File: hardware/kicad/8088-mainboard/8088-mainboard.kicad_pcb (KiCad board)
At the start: 2 copper layers, 149 x 90 mm, 62 parts, among them J1 Exp0, J2 POWER 5v, J3 Exp1, J4 Exp2, SW1 Reset, U1 8088, U10 74LS273, U11 74LS00, U12 74LS138, U13 HM62256BLP, U2 8284, U3 74LS373, U4 74LS373, U5 74LS245, U6 8288, U7 74LS138, U8 28C256, U9 HM62256BLP, Y1 14.31818 MHz

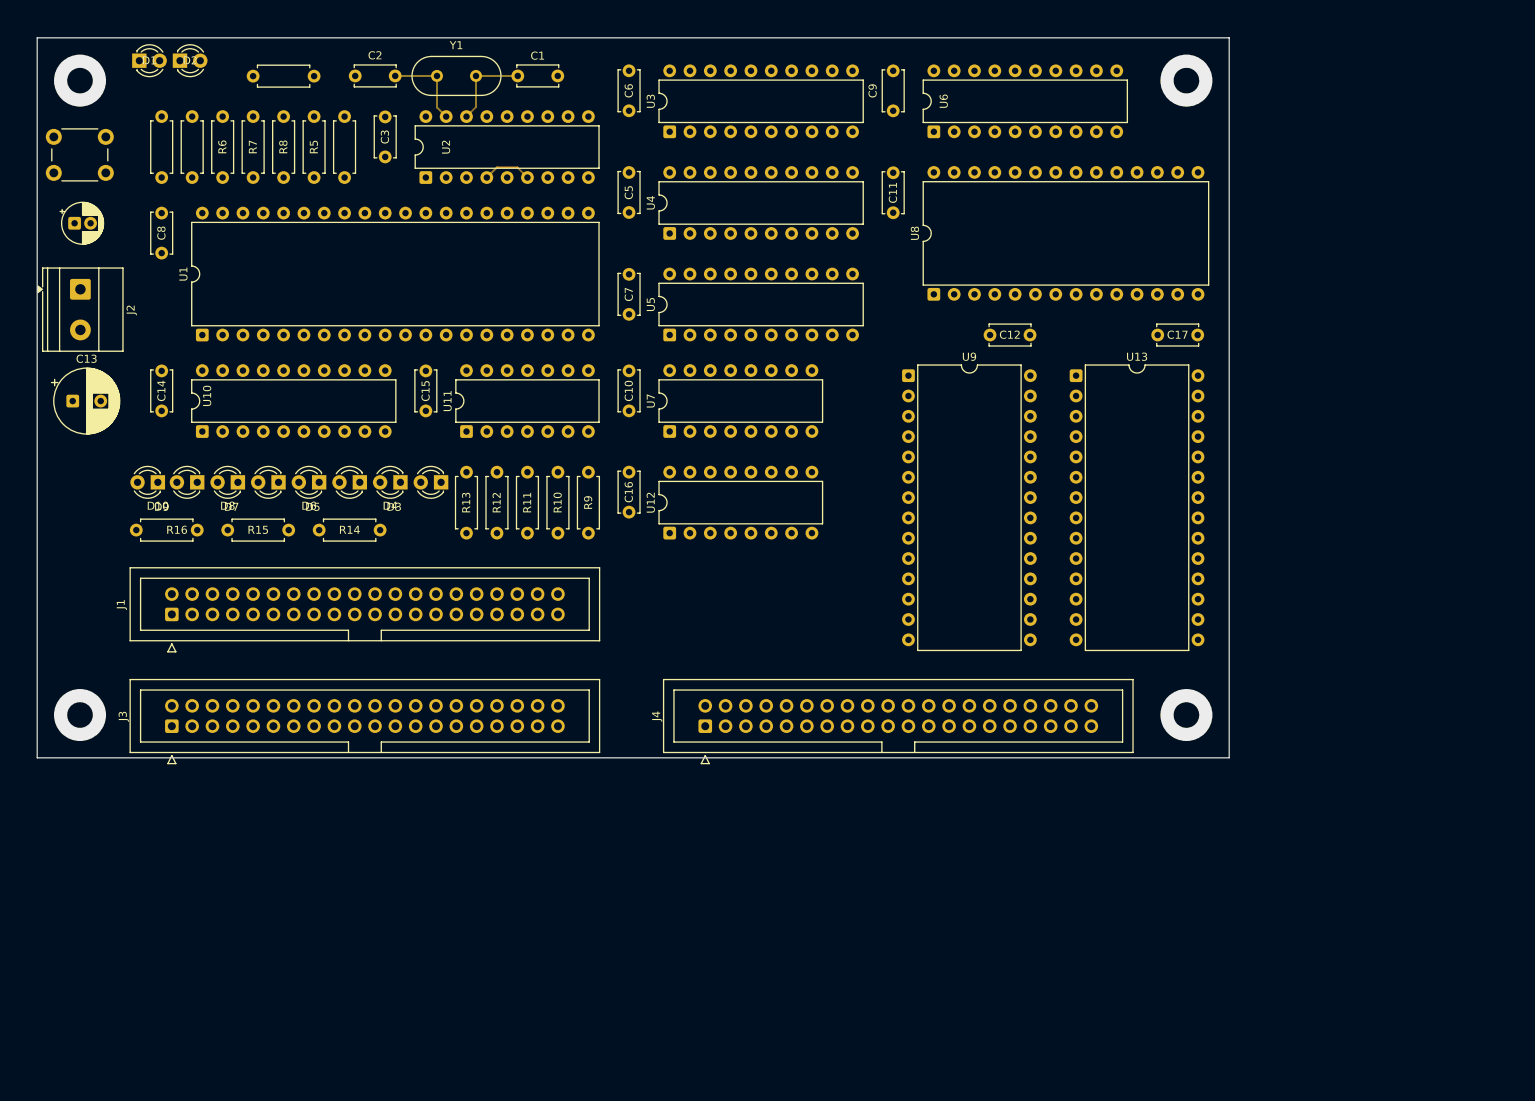
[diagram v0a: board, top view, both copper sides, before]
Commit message: Add PSB board design
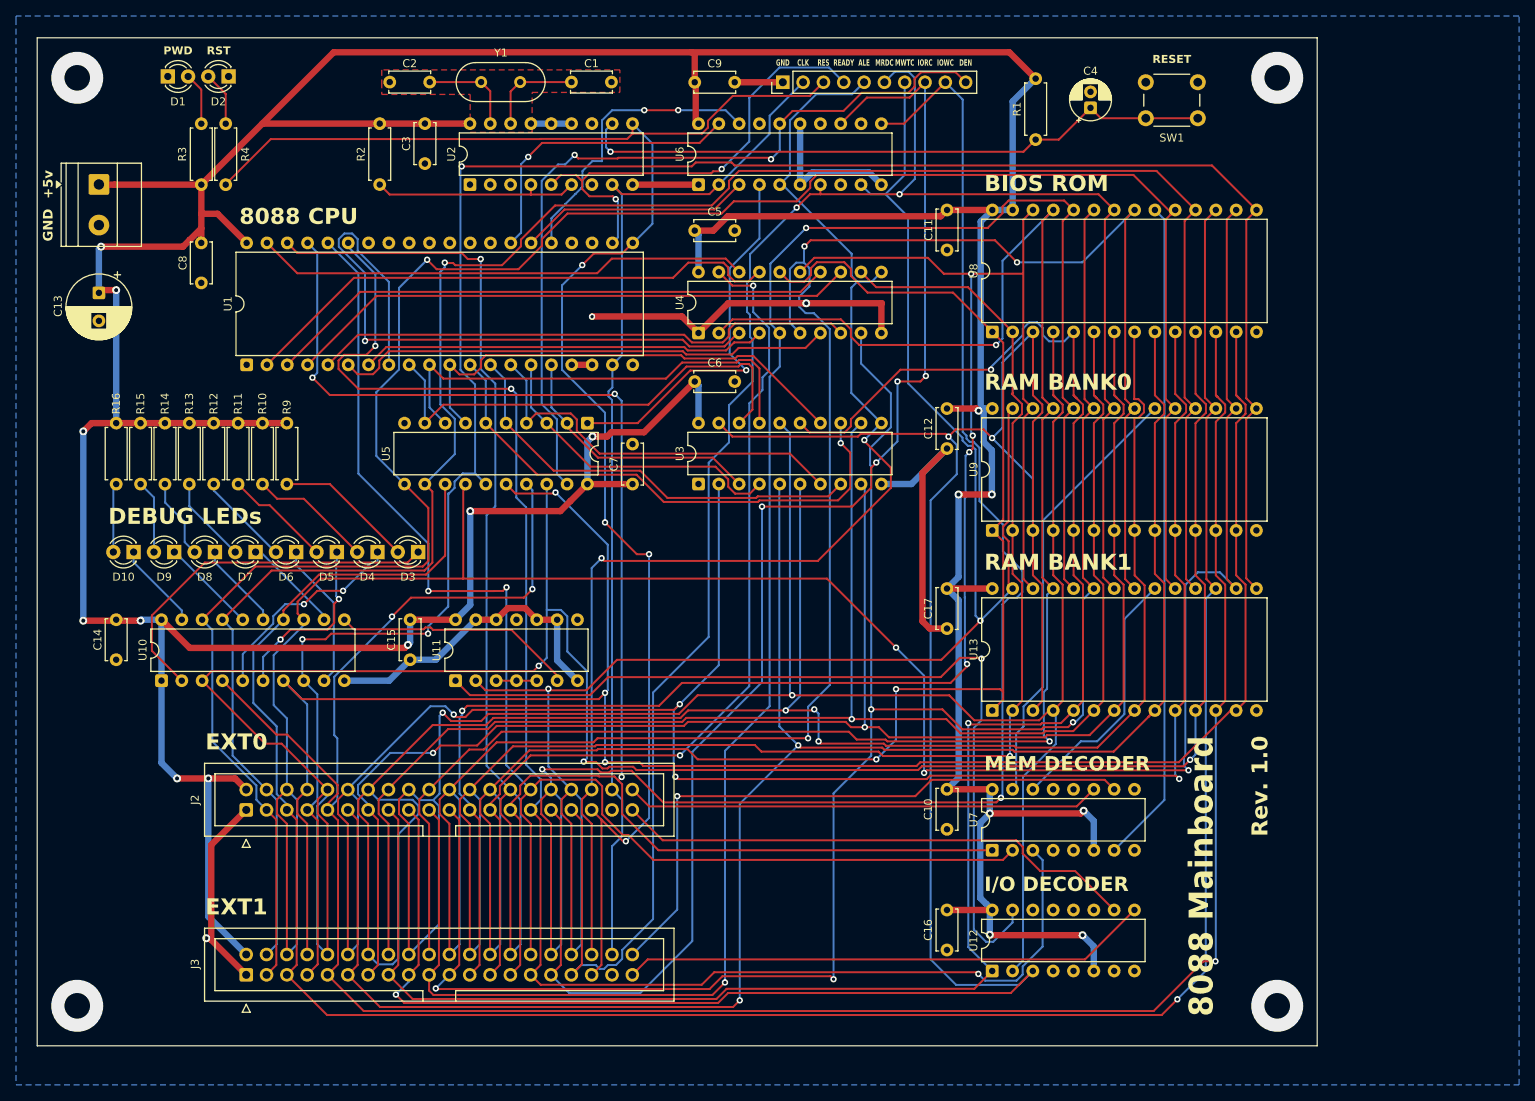
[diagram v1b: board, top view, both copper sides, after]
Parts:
- removed J4: Exp2, Connector_IDC:IDC-Header_2x20_P2.54mm_Vertical
- removed R5, R6, R7, R8: 10k, Resistor_THT:R_Axial_DIN0207_L6.3mm_D2.5mm_P7.62mm_Horizontal
- added J_DEBUG1: DEBUG, Connector_PinHeader_2.54mm:PinHeader_1x10_P2.54mm_Vertical, F.Cu at (113.2, 25.6)
- moved SW1 143.0 mm to (165.1, 30.1), turned to 180 degrees
- moved C4 127.8 mm to (151.7, 28.8), turned to 90 degrees
- moved R1 106.2 mm to (144.8, 25.1), turned to -90 degrees
- moved U12 68.0 mm to (139.4, 136.6)
- moved C16 67.6 mm to (133.7, 129.0)
- moved U7 66.1 mm to (139.4, 121.6)
- moved C10 65.7 mm to (133.7, 113.9)
- moved C17 44.6 mm to (133.7, 88.8), turned to -90 degrees
- moved U3 44.2 mm to (102.7, 75.8)
- moved U13 43.1 mm to (139.4, 104.1), turned to 90 degrees
- moved R9 40.1 mm to (51.2, 68.2), turned to -90 degrees
- moved C6 39.7 mm to (102.2, 63.0), turned to 0 degrees
- moved R10 39.4 mm to (48.2, 68.2), turned to -90 degrees
- moved R11 38.7 mm to (45.1, 68.2), turned to -90 degrees
- moved R12 38.0 mm to (42.1, 68.2), turned to -90 degrees
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- renumbered J2 to J1, J1 to J2
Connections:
- J2 pad 1: VCC -> GND
- J2 pad 10: /A7 -> /D0
- J2 pad 11: /A8 -> /A1
- J2 pad 12: /A9 -> /A0
- J2 pad 13: /A10 -> /A3
- J2 pad 14: /A11 -> /A2
- J2 pad 15: /A12 -> /A5
- J2 pad 16: /A13 -> /A4
- J2 pad 17: /A14 -> /A7
- J2 pad 18: /A15 -> /A6
- J2 pad 19: /A16 -> /A9
- J2 pad 2: GND -> VCC
- J2 pad 20: /A17 -> /A8
- J2 pad 21: /A18 -> /A11
- J2 pad 22: /A19 -> /A10
- J2 pad 23: /D0 -> /A13
- J2 pad 24: /D1 -> /A12
- J2 pad 25: /D2 -> /A15
- J2 pad 26: /D3 -> /A14
- J2 pad 27: /D4 -> /A17
- J2 pad 28: /D5 -> /A16
- J2 pad 29: /D6 -> /A19
- J2 pad 3: /A0 -> /D7
- J2 pad 30: /D7 -> /A18
- J2 pad 31: /MRDC -> /IORC
- J2 pad 32: /MWTC -> /IOWC
- J2 pad 33: /IORC -> /MRDC
- J2 pad 34: /IOWC -> /MWTC
- J2 pad 35: /MEM_DECODER/MEM_80000_9FFFF -> /RESET
- J2 pad 36: /IO_DECODER/IO_A0_BF -> /ALE
- J2 pad 37: /CLK -> GND
- J2 pad 38: /ALE -> /CLK
- J2 pad 39: /RESET -> /IO_DECODER/IO_A0_BF
- J2 pad 4: /A1 -> /D6
- J2 pad 40: GND -> /MEM_DECODER/MEM_80000_9FFFF
- J2 pad 5: /A2 -> /D5
- J2 pad 6: /A3 -> /D4
- J2 pad 7: /A4 -> /D3
- J2 pad 8: /A5 -> /D2
- J2 pad 9: /A6 -> /D1
- J3 pad 1: VCC -> GND
- J3 pad 10: /A7 -> /D0
- J3 pad 11: /A8 -> /A1
- J3 pad 12: /A9 -> /A0
- J3 pad 13: /A10 -> /A3
- J3 pad 14: /A11 -> /A2
- J3 pad 15: /A12 -> /A5
- J3 pad 16: /A13 -> /A4
- J3 pad 17: /A14 -> /A7
- J3 pad 18: /A15 -> /A6
- J3 pad 19: /A16 -> /A9
- J3 pad 2: GND -> VCC
- J3 pad 20: /A17 -> /A8
- J3 pad 21: /A18 -> /A11
- J3 pad 22: /A19 -> /A10
- J3 pad 23: /D0 -> /A13
- J3 pad 24: /D1 -> /A12
- J3 pad 25: /D2 -> /A15
- J3 pad 26: /D3 -> /A14
- J3 pad 27: /D4 -> /A17
- J3 pad 28: /D5 -> /A16
- J3 pad 29: /D6 -> /A19
- J3 pad 3: /A0 -> /D7
- J3 pad 30: /D7 -> /A18
- J3 pad 31: /MRDC -> /IORC
- J3 pad 32: /MWTC -> /IOWC
- J3 pad 33: /IORC -> /MRDC
- J3 pad 34: /IOWC -> /MWTC
- J3 pad 35: /MEM_DECODER/MEM_A0000_BFFFF -> /RESET
- J3 pad 36: /IO_DECODER/IO_C0_DF -> /ALE
- J3 pad 37: /CLK -> GND
- J3 pad 38: /ALE -> /CLK
- J3 pad 39: /RESET -> /IO_DECODER/IO_C0_DF
- J3 pad 4: /A1 -> /D6
- J3 pad 40: GND -> /MEM_DECODER/MEM_A0000_BFFFF
- J3 pad 5: /A2 -> /D5
- J3 pad 6: /A3 -> /D4
- J3 pad 7: /A4 -> /D3
- J3 pad 8: /A5 -> /D2
- J3 pad 9: /A6 -> /D1
- U1 pad 17: Net-(U1-NMI) -> GND
- U1 pad 18: Net-(U1-INTR) -> GND
- U1 pad 23: Net-(U1-~{TEST}) -> GND
- U1 pad 31: Net-(U1-HOLD) -> GND
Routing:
- net VCC: track 0.00 -> 651.2 mm, vias 0 -> 17
- net /A7: track 0.00 -> 303.5 mm, vias 0 -> 3
- net /D1: track 0.00 -> 302.2 mm, vias 0 -> 3
- net /D5: track 0.00 -> 299.6 mm, vias 0 -> 1
- net /D4: track 0.00 -> 292.5 mm, vias 0 -> 3
- net /D0: track 0.00 -> 286.5 mm, vias 0 -> 3
- net /D3: track 0.00 -> 277.1 mm, vias 0 -> 3
- net /D7: track 0.00 -> 274.6 mm, vias 0 -> 1
- net /D6: track 0.00 -> 266.9 mm, vias 0 -> 1
- net /A10: track 0.00 -> 262.5 mm, vias 0 -> 3
- net /A6: track 0.00 -> 257.2 mm, vias 0 -> 2
- net /A11: track 0.00 -> 254.8 mm, vias 0 -> 4
- net /D2: track 0.00 -> 253.1 mm, vias 0 -> 3
- net /A0: track 0.00 -> 251.7 mm, vias 0 -> 4
- net /A9: track 0.00 -> 247.0 mm, vias 0 -> 2
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- added copper zone on B.Cu, net GND
- added copper zone on F.Cu, net GND
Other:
- board size 149 x 90 mm -> 160 x 126 mm
- board text added: "+5v"
- board text added: "8088 CPU"
- board text added: "8088 Mainboard"
- board text added: "ALE"
- board text added: "BIOS ROM"
- board text added: "CLK"
- board text added: "DEBUG LEDs"
- board text added: "DEN"
- board text added: "EXT0"
- board text added: "EXT1"
- board text added: "GND"
- board text added: "I/O DECODER"
- board text added: "IORC"
- board text added: "IOWC"
- board text added: "MEM DECODER"
- board text added: "MRDC"
- board text added: "MWTC"
- board text added: "PWD"
- board text added: "Project: github.com/i-melnichenko/8088-homebrew-computer"
- board text added: "RAM BANK0"
- board text added: "RAM BANK1"
- board text added: "READY"
- board text added: "RES"
- board text added: "RESET"
- board text added: "RST"
- board text added: "Rev. 1.0"
